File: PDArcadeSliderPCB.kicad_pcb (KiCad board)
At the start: 2 copper layers, 100 x 63.6 mm, 28 parts, among them J1 Conn_01x01_Male, J2 Conn_01x06_Male, J6 Conn_01x01_Male, J7 Conn_01x01_Male, J8 Conn_01x01_Male, J9 Conn_01x01_Male, U1 testsensorg, U2 testsensorg, U3 testsensorg, U4 testsensorg, U5 testsensorg, U6 testsensorg

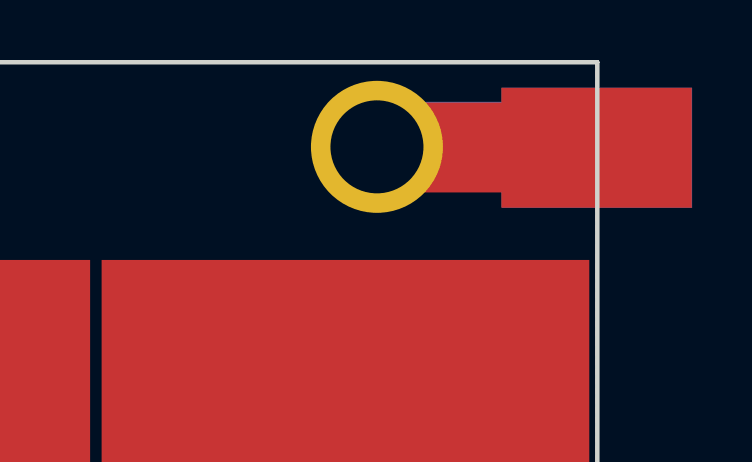
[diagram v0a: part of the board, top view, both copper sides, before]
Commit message: Update PDArcadeSliderPCB.kicad_pcb
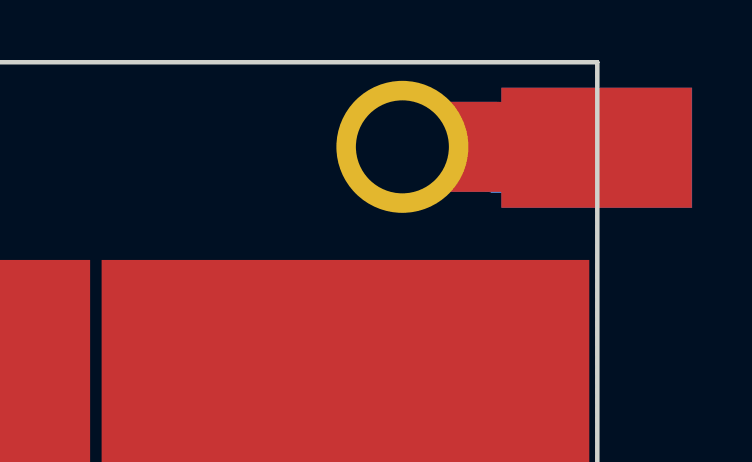
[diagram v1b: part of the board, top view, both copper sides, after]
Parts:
- moved REF** 0.85 mm to (193.6, 108.0)
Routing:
- net GND: track 35.9 -> 34.3 mm
